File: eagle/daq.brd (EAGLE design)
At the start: 59.7 x 65.4 mm, 80 parts

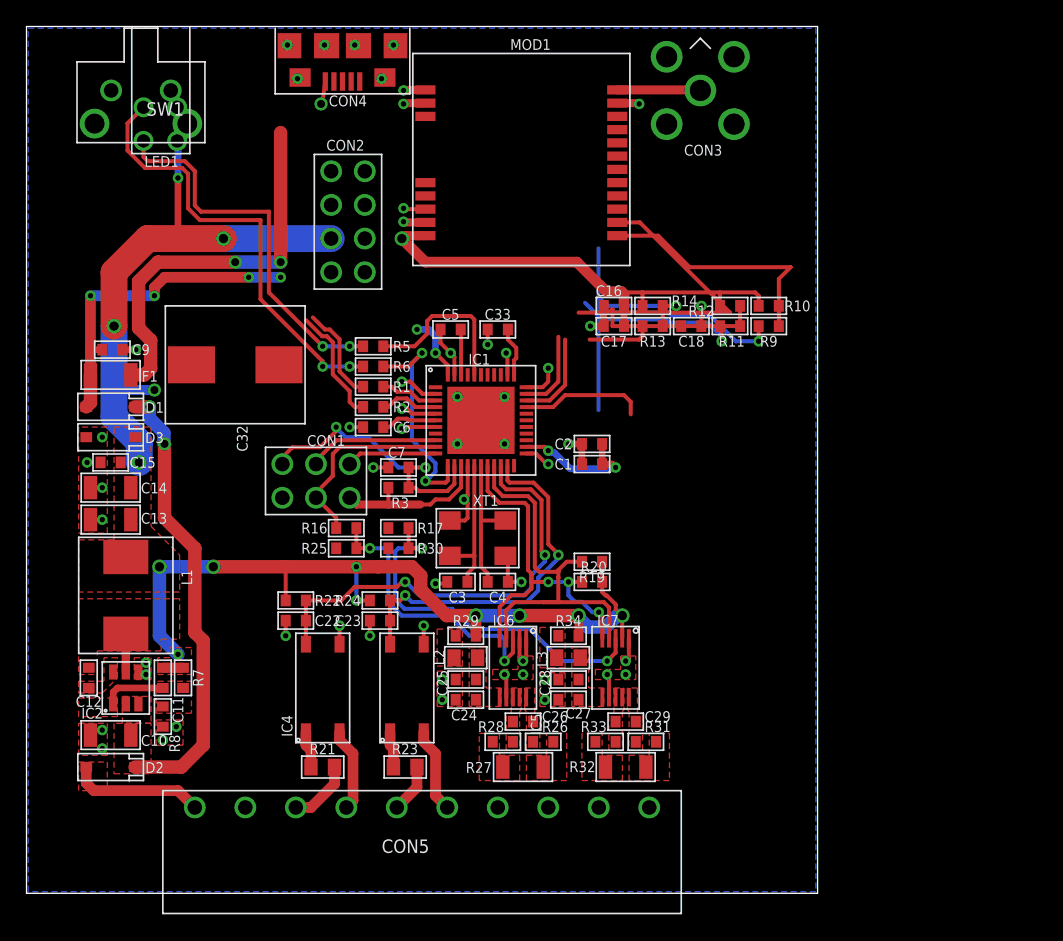
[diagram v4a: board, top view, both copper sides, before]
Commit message: do
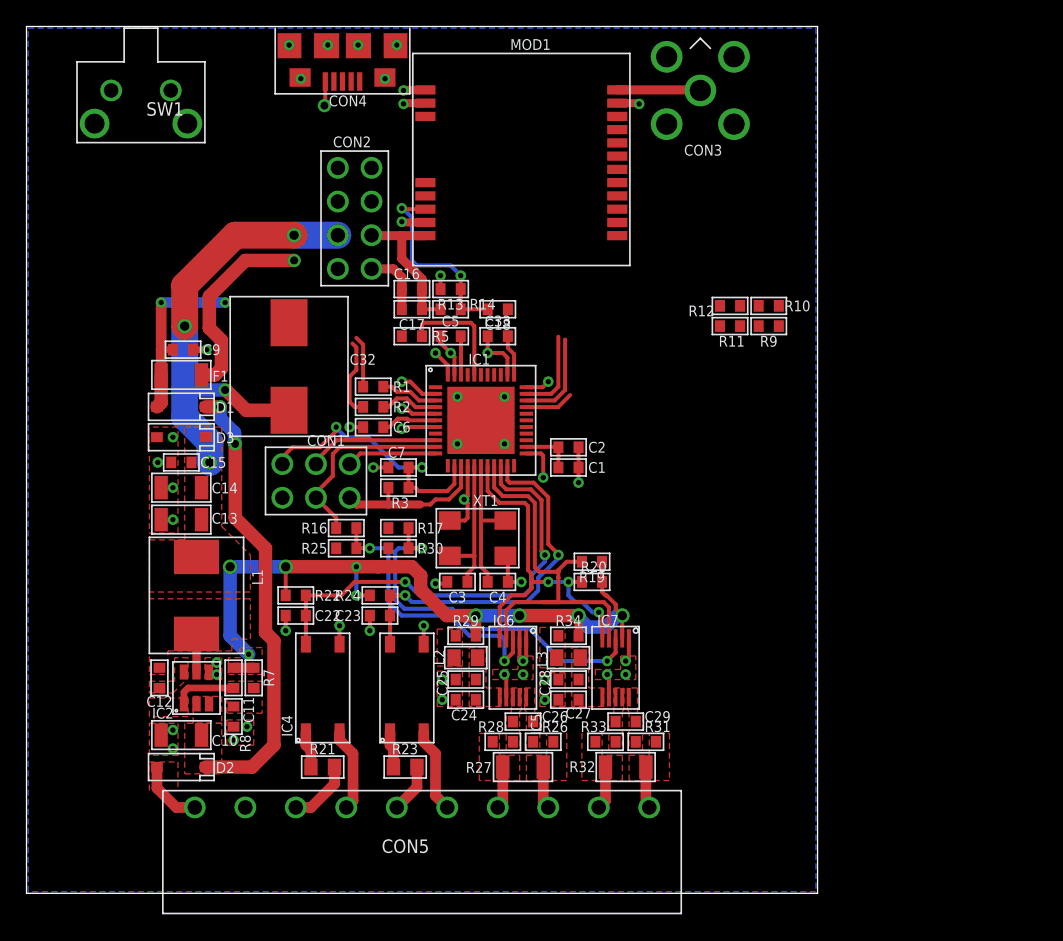
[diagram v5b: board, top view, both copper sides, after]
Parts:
- removed LED1: (no value), myparts:LED-HOLDER-2P
- removed R6: (no value), myparts:0603
- moved R13 15.5 mm to (32.0, 45.6)
- moved C16 15.3 mm to (29.1, 45.6)
- moved C17 15.3 mm to (29.1, 44.1)
- moved R14 15.2 mm to (32.0, 44.1)
- moved C18 14.7 mm to (35.6, 44.1)
- moved C10 5.33 mm to (11.7, 11.9)
- moved C11 5.33 mm to (15.6, 16.3)
- moved C12 5.33 mm to (10.0, 16.3)
- moved C13 5.33 mm to (11.7, 28.2)
- moved C14 5.33 mm to (11.7, 30.6)
- moved C15 5.33 mm to (11.7, 32.5)
- moved C9 5.33 mm to (11.8, 41.0)
- moved D1 5.33 mm to (11.7, 36.7)
- moved D2 5.33 mm to (11.7, 9.53)
- moved D3 5.33 mm to (11.7, 34.4)
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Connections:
- removed net N$15: LED1.3, R5.2
- removed net N$30: CON5.9, R31.1, R32.1
- removed net N$36: IC1.12, R6.1
- net N$40: now also R31.1, R32.1; no longer R32.2, R33.1
- net N$59: now also R27.1, R28.2; no longer R26.2, R27.2
- net N$8: now also CON5.9, R32.2, R33.1; no longer LED1.1, R6.2
- net N$81: now also R26.2, R27.2; no longer R27.1, R28.2
- net VCC: no longer LED1.2, LED1.4
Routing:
- net N$7: track 35.6 -> 0.00 mm
- net N$8: track 33.5 -> 3.26 mm, vias 2 -> 0
- net N$15: track 28.8 -> 0.00 mm, vias 2 -> 0
- net VCC: track 139.0 -> 113.4 mm, vias 18 -> 14
- net N$13: track 36.1 -> 11.7 mm, vias 1 -> 0
- net N$6: track 18.9 -> 0.00 mm
- net N$14: track 18.7 -> 0.00 mm, vias 1 -> 0
- net N$36: track 17.3 -> 0.00 mm, vias 2 -> 0
- net N$56: track 29.8 -> 15.0 mm, vias 2 -> 1
- net N$16: track 12.9 -> 0.18 mm, vias 1 -> 0
- net UVCC: track 30.2 -> 19.2 mm, vias 6 -> 4
- net N$22: track 14.3 -> 4.69 mm, vias 0 -> 1
- net N$2: track 20.3 -> 14.8 mm
- net VEXT: track 10.2 -> 5.05 mm
- net N$1: track 12.7 -> 8.67 mm
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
